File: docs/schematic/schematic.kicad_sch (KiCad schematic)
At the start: 8 parts, among them J1 RJ45, U1 CCGM1A1, U2 SP3485EN, U3 SP3485EN

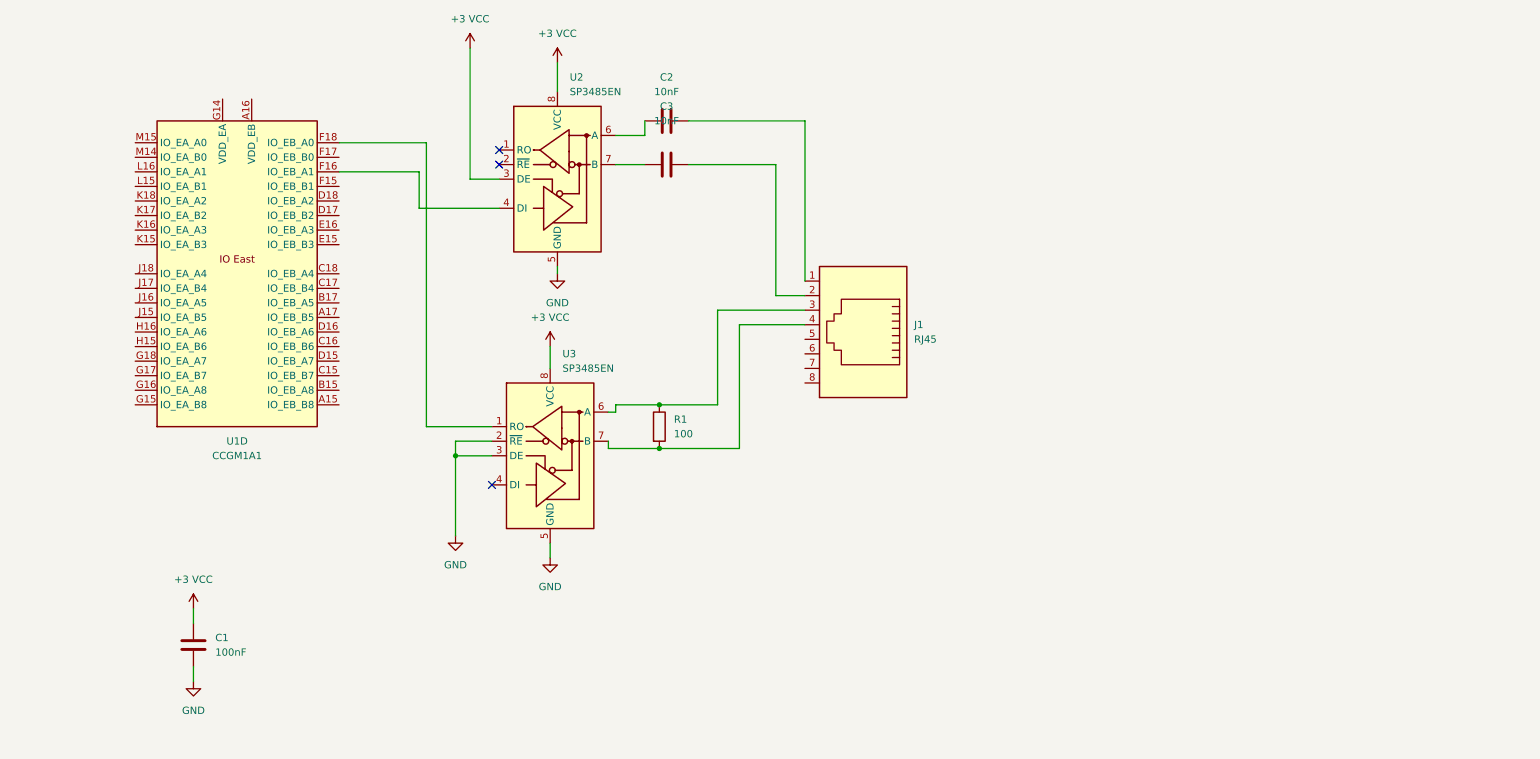
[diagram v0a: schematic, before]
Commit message: Updated schematics
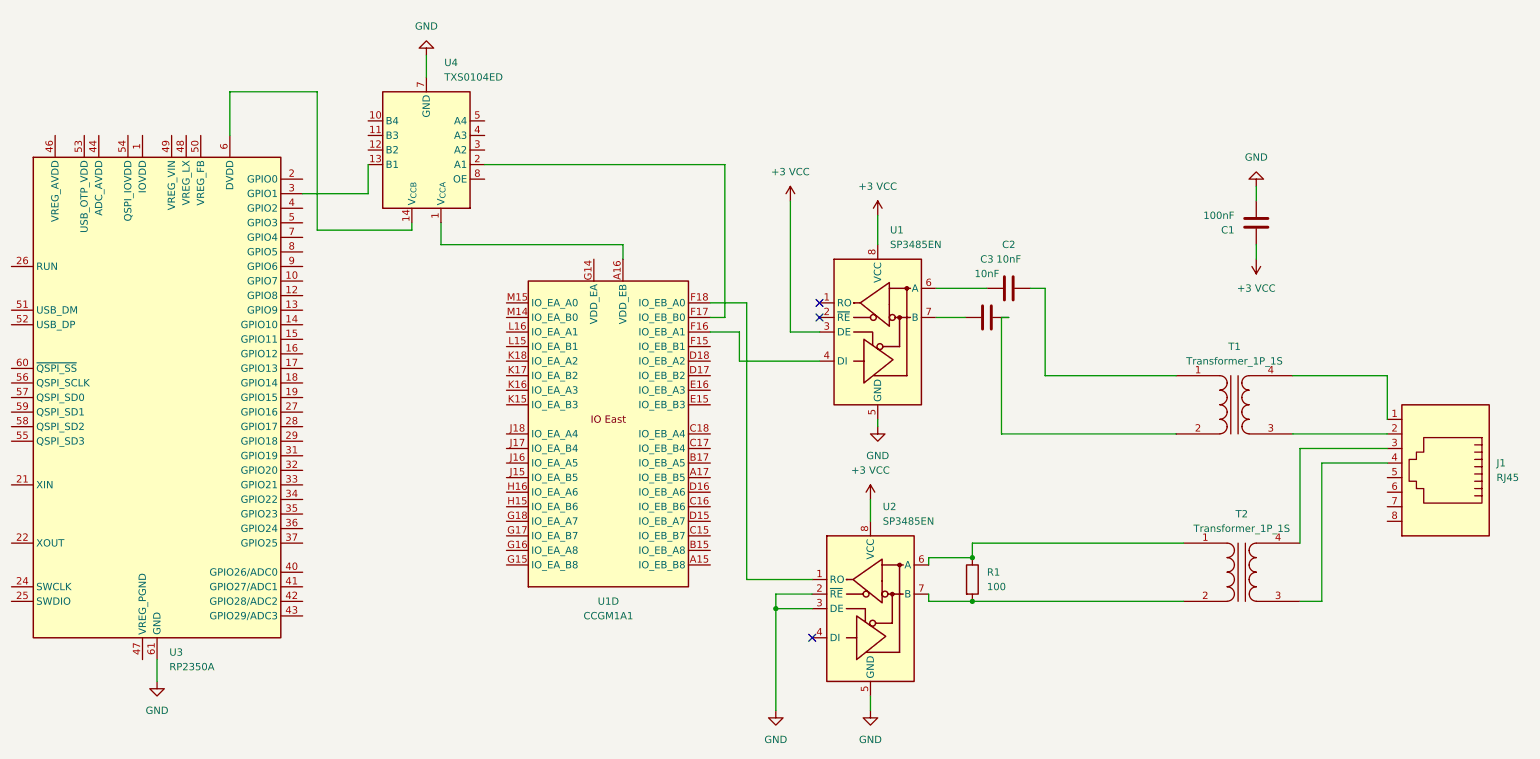
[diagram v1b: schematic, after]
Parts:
- added T1, T2: Transformer_1P_1S, symbol Device:Transformer_1P_1S
- added U3: RP2350A, Package_DFN_QFN:QFN-60-1EP_7x7mm_P0.4mm_EP3.4x3.4mm, symbol MCU_RaspberryPi:RP2350A
- added U4: TXS0104ED, Package_SO:SOIC-14_3.9x8.7mm_P1.27mm, symbol Logic_LevelTranslator:TXS0104ED
- renumbered U2 to U1, U3 to U2
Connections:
- net GND: now also U3.61 (GND), U4.7 (GND)
- net at R1.1, U2.6 (A): now also T2.1 (AA); no longer J1.3
- net at R1.2, U2.7 (B): now also T2.2 (AB); no longer J1.4
- net at C3.2: now also T1.2 (AB); no longer J1.2
- net at U1.A16 (VDD_EB), U1.B18 (VDD_EB), U1.E14 (VDD_EB)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: now also U4.1 (V_{CCA})
- net at U1.F17 (IO_EB_B0): now also U4.2 (A1)
- net at C2.2: now also T1.1 (AA); no longer J1.1
- new net: J1.2, T1.3 (SA)
- new net: J1.1, T1.4 (SB)
- new net: U3.1 (IOVDD), U3.11 (IOVDD), U3.20 (IOVDD), U3.30 (IOVDD), U3.38 (IOVDD), U3.45 (IOVDD)
- new net: U3.23 (DVDD), U3.39 (DVDD), U3.6 (DVDD), U4.14 (V_{CCB})
- new net: U3.3 (GPIO1), U4.13 (B1)
- new net: J1.4, T2.3 (SA)
- new net: J1.3, T2.4 (SB)
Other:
- moved on the sheet: C1, C2, C3, J1, U1, U1D, U2
